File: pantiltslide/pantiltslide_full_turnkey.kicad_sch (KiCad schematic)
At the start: 57 parts, among them J1 Conn_01x22_Socket, J17 Motor_Slide, J18 Motor_Pan, J19 Motor_Tilt, J2 Conn_01x22_Socket, J20 TCA9548A_Mux, J21 AS5600_Pan, J22 AS5600_Tilt, J23 OLED, J24 TCA9548A_Mux, J26 Limit_Min, J27 Limit_Max, J28 Motor_Aux, J29 Enc_Slide, J30 Enc_Pan, J31 Enc_Tilt, J32 Enc_Aux, J33 Btn_SetKeyframe, J34 Btn_ClearKeyframe, J35 Btn_PlayPause, J36 Btn_Reset, J37 5V_In, J38 24V_In, J41 Aux_Max, U1 tmc2209, U2 tmc2209, U3 tmc2209, U4 tmc2209

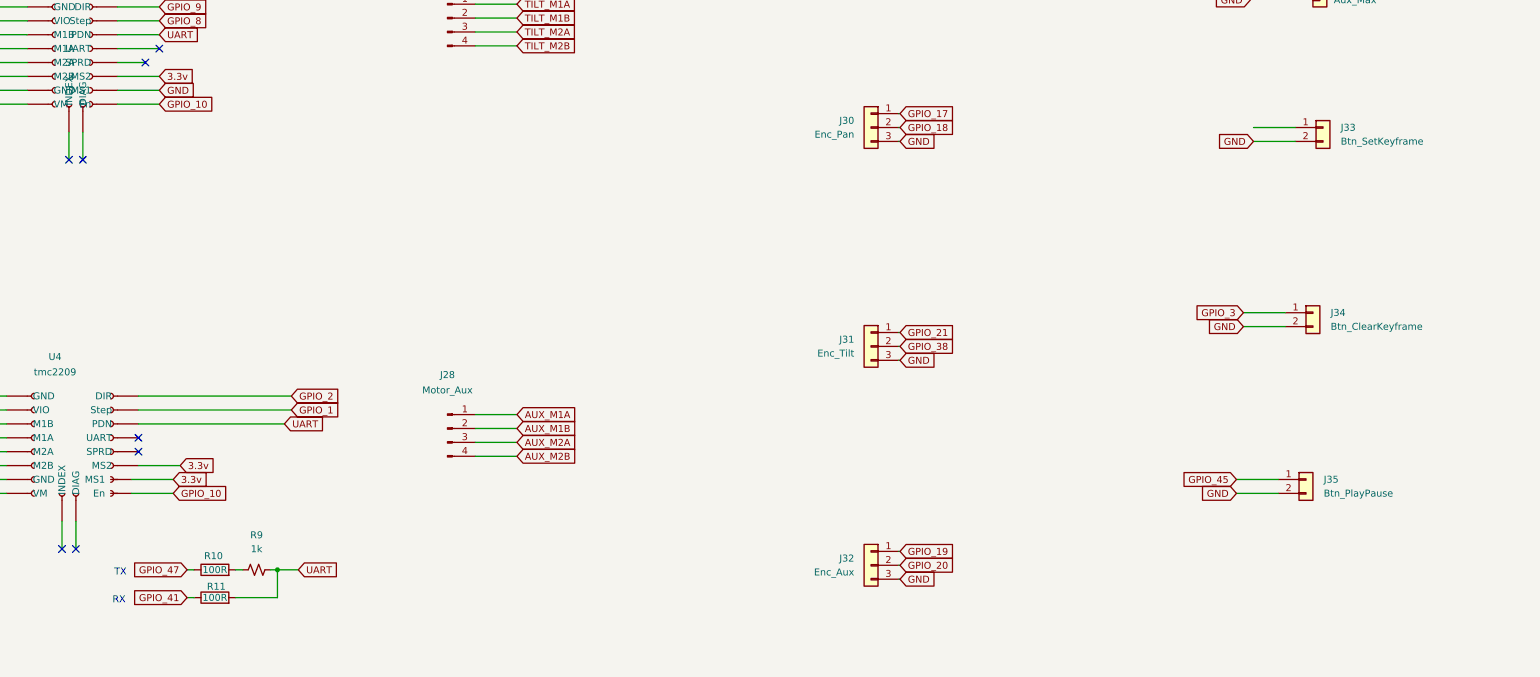
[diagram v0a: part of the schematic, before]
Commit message: more corrections and refinements before prod
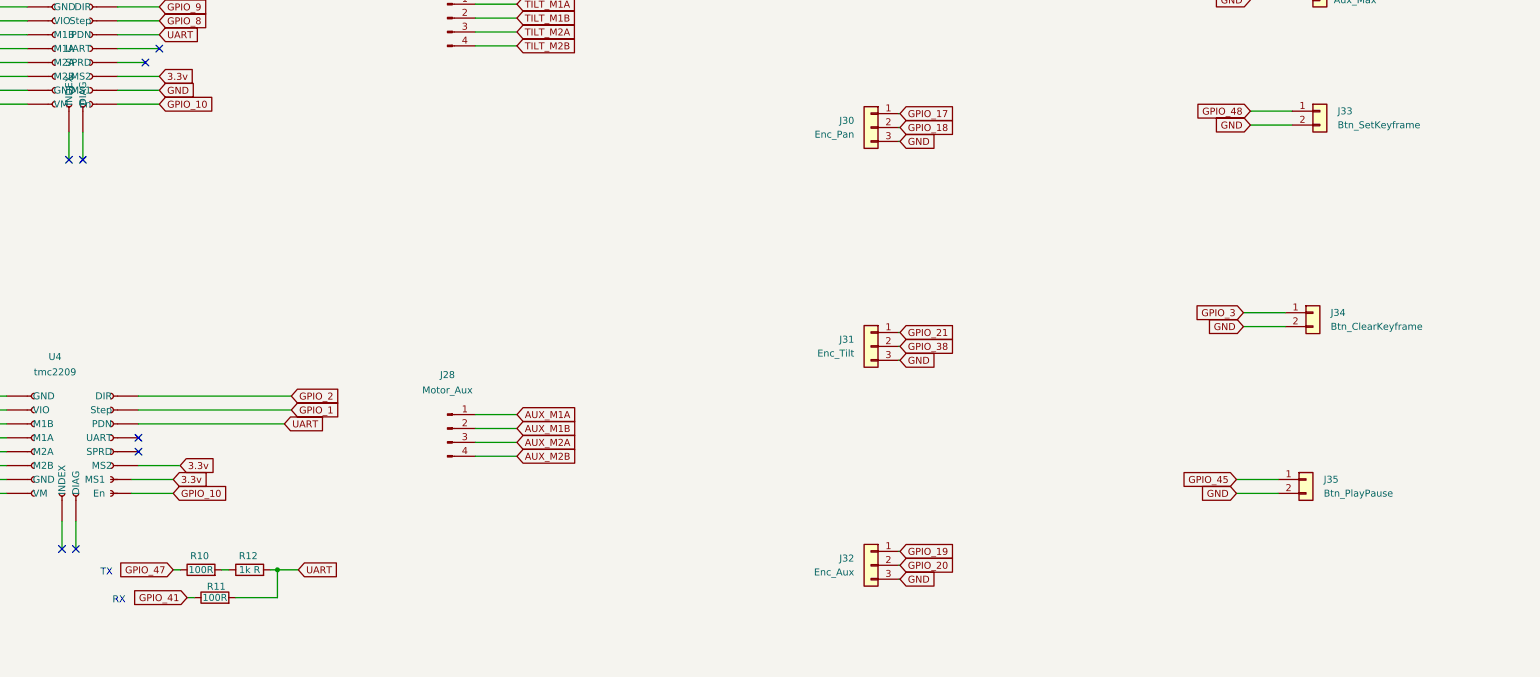
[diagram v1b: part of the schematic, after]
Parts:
- removed R9: 1k, PCM_SparkFun-Resistor:R_0402_1005Metric, symbol PCM_SparkFun-Resistor:1k_0402
- added R12: 1k R, Resistor_SMD:R_0603_1608Metric, symbol Device:R
- R10, R11: footprint (none) -> Resistor_SMD:R_0603_1608Metric
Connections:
- net GPIO_48: now also J33.1 (Pin_1)
- net UART: now also R12.2
- net at R10.2: now also R12.1
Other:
- moved on the sheet: J33, R10
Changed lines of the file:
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@@
 	(text "TX\n"
 		(exclude_from_sim no)
-		(at 300.228 291.338 0)
+		(at 297.688 291.338 0)
 		(effects
 			(font
@@
 	)
 	(junction
+		(at 328.93 290.83)
+		(diameter 0)
+		(color 0 0 0 0)
+	)
+	(junction
 		(at 123.19 345.44)
 		(diameter 0)
@@
 	)
 	(junction
-		(at 328.93 290.83)
-		(diameter 0)
-		(color 0 0 0 0)
-	)
-	(junction
 		(at 59.69 345.44)
 		(diameter 0)
@@
 	(wire
 		(pts
-			(xy 514.92 212.54) (xy 507.3 212.54)
+			(xy 514.35 209.55) (xy 506.73 209.55)
 		)
 		(stroke
@@
 	(wire
 		(pts
-			(xy 514.92 210) (xy 507.3 210)
+			(xy 514.35 207.01) (xy 506.73 207.01)
 		)
 		(stroke
@@
 	(wire
 		(pts
+			(xy 327.66 290.83) (xy 328.93 290.83)
+		)
+		(stroke
+			(width 0)
+			(type default)
+		)
+	)
+	(wire
+		(pts
 			(xy 116.84 96.52) (xy 130.81 96.52)
 		)
@@
 	(wire
 		(pts
+			(xy 318.77 290.83) (xy 320.04 290.83)
+		)
+		(stroke
+			(width 0)
+			(type default)
+		)
+	)
+	(wire
+		(pts
 			(xy 365.08 115) (xy 372.7 115)
 		)
@@
 	(wire
 		(pts
-			(xy 312.42 290.83) (xy 313.69 290.83)
+			(xy 309.88 290.83) (xy 311.15 290.83)
 		)
 		(stroke
@@
 	(wire
 		(pts
-			(xy 322.58 290.83) (xy 321.31 290.83)
-		)
-		(stroke
-			(width 0)
-			(type default)
-		)
-	)
-	(wire
-		(pts
 			(xy 299.72 118.11) (xy 307.34 118.11)
 		)
@@
 		)
 	)
-	(wire
-		(pts
-			(xy 327.66 290.83) (xy 328.93 290.83)
-		)
-		(stroke
-			(width 0)
-			(type default)
-		)
-	)
 	(label "A1"
 		(at 514.35 41.91 180)
@@
 	(global_label "GPIO_47"
 		(shape input)
-		(at 312.42 290.83 180)
+		(at 309.88 290.83 180)
 		(effects
 			(font
@@
 		)
 		(property "Intersheetrefs" "${INTERSHEET_REFS}"
-			(at 312.42 290.83 0)
+			(at 309.88 290.83 0)
 			(hide yes)
 			(show_name no)
@@
 	(global_label "GND"
 		(shape input)
-		(at 507.3 212.54 180)
+		(at 506.73 209.55 180)
 		(effects
 			(font
@@
 		)
 		(property "Intersheetrefs" "${INTERSHEET_REFS}"
-			(at 507.3 212.54 0)
+			(at 506.73 209.55 0)
 			(hide yes)
 			(show_name no)
@@
 		)
 	)
+	(global_label "GPIO_48"
+		(shape input)
+		(at 506.73 207.01 180)
+		(effects
+			(font
+				(size 1.27 1.27)
+			)
+			(justify right)
+		)
+		(property "Intersheetrefs" "${INTERSHEET_REFS}"
+			(at 506.73 207.01 0)
+			(hide yes)
+			(show_name no)
+			(do_not_autoplace no)
+			(effects
+				(font
+					(size 1.27 1.27)
+				)
+			)
+		)
+	)
 	(global_label "MUX_CH4_SCL"
 		(shape input)
@@
 			)
 		)
-		(property "Footprint" ""
+		(property "Footprint" "Resistor_SMD:R_0603_1608Metric"
 			(at 317.5 297.688 90)
 			(hide yes)
@@
 	)
 	(symbol
-		(lib_id "PCM_SparkFun-Resistor:1k_0402")
-		(at 325.12 290.83 0)
-		(unit 1)
-		(body_style 1)
-		(exclude_from_sim no)
-		(in_bom yes)
-		(on_board yes)
-		(in_pos_files yes)
-		(dnp no)
-		(fields_autoplaced yes)
-		(property "Reference" "R9"
-			(at 325.12 284.48 0)
-			(show_name no)
-			(do_not_autoplace no)
-			(effects
-				(font
-					(size 1.27 1.27)
-				)
-			)
-		)
-		(property "Value" "1k"
-			(at 325.12 287.02 0)
-			(show_name no)
-			(do_not_autoplace no)
-			(effects
-				(font
-					(size 1.27 1.27)
-				)
-			)
-		)
-		(property "Footprint" "PCM_SparkFun-Resistor:R_0402_1005Metric"
-			(at 325.12 295.402 0)
-			(hide yes)
-			(show_name no)
-			(do_not_autoplace no)
-			(effects
-				(font
-					(size 1.27 1.27)
-				)
-			)
-		)
-		(property "Datasheet" "https://www.vishay.com/docs/20035/dcrcwe3.pdf"
-			(at 323.85 299.72 0)
-			(hide yes)
-			(show_name no)
-			(do_not_autoplace no)
-			(effects
-				(font
-					(size 1.27 1.27)
-				)
-			)
-		)
-		(property "Description" "Resistor"
-			(at 325.12 302.26 0)
-			(hide yes)
-			(show_name no)
-			(do_not_autoplace no)
-			(effects
-				(font
-					(size 1.27 1.27)
-				)
-			)
-		)
-		(property "PROD_ID" "RES-14342"
-			(at 325.12 297.688 0)
-			(hide yes)
-			(show_name no)
-			(do_not_autoplace no)
-			(effects
-				(font
-					(size 1.27 1.27)
-				)
-			)
-		)
-		(pin "2"
-		)
-		(pin "1"
-		)
-		(instances
-			(project "pantiltslide_full_turnkey"
-				(path "/069dac62-ca78-4a21-b689-b9421532705f"
-					(reference "R9")
-					(unit 1)
-				)
-			)
-		)
-	)
-	(symbol
 		(lib_id "Connector_Generic:Conn_01x03")
 		(at 437.41 170 0)
@@
 	)
 	(symbol
+		(lib_id "Device:R")
+		(at 323.85 290.83 90)
+		(unit 1)
+		(body_style 1)
+		(exclude_from_sim no)
+		(in_bom yes)
+		(on_board yes)
+		(in_pos_files yes)
+		(dnp no)
+		(property "Reference" "R12"
+			(at 323.596 288.29 90)
+			(show_name no)
+			(do_not_autoplace no)
+			(effects
+				(font
+					(size 1.27 1.27)
+				)
+			)
+		)
+		(property "Value" "1k R"
+			(at 323.85 290.83 90)
+			(show_name no)
+			(do_not_autoplace no)
+			(effects
+				(font
+					(size 1.27 1.27)
+				)
+			)
+		)
+		(property "Footprint" "Resistor_SMD:R_0603_1608Metric"
+			(at 323.85 292.608 90)
+			(hide yes)
+			(show_name no)
+			(do_not_autoplace no)
+			(effects
+				(font
+					(size 1.27 1.27)
+				)
+			)
+		)
+		(property "Datasheet" ""
+			(at 323.85 290.83 0)
+			(hide yes)
+			(show_name no)
+			(do_not_autoplace no)
+			(effects
+				(font
+					(size 1.27 1.27)
+				)
+			)
+		)
+		(property "Description" "Resistor"
+			(at 323.85 290.83 0)
+			(hide yes)
+			(show_name no)
+			(do_not_autoplace no)
+			(effects
+				(font
+					(size 1.27 1.27)
+				)
+			)
+		)
+		(pin "1"
+		)
+		(pin "2"
+		)
+		(instances
+			(project "pantiltslide_full_turnkey"
+				(path "/069dac62-ca78-4a21-b689-b9421532705f"
+					(reference "R12")
+					(unit 1)
+				)
+			)
+		)
+	)
+	(symbol
 		(lib_id "power:GND")
 		(at 144.78 382.27 0)
@@
 	(symbol
 		(lib_id "Device:R")
-		(at 317.5 290.83 90)
+		(at 314.96 290.83 90)
 		(unit 1)
 		(body_style 1)
@@
 		(dnp no)
 		(property "Reference" "R10"
-			(at 317.246 288.29 90)
+			(at 314.706 288.29 90)
 			(show_name no)
 			(do_not_autoplace no)
@@
 		)
 		(property "Value" "100R"
-			(at 317.5 290.83 90)
+			(at 314.96 290.83 90)
 			(show_name no)
 			(do_not_autoplace no)
@@
 			)
 		)
-		(property "Footprint" ""
-			(at 317.5 292.608 90)
+		(property "Footprint" "Resistor_SMD:R_0603_1608Metric"
+			(at 314.96 292.608 90)
 			(hide yes)
 			(show_name no)
@@
 		)
 		(property "Datasheet" ""
-			(at 317.5 290.83 0)
+			(at 314.96 290.83 0)
 			(hide yes)
 			(show_name no)
@@
 		)
 		(property "Description" "Resistor"
-			(at 317.5 290.83 0)
+			(at 314.96 290.83 0)
 			(hide yes)
 			(show_name no)
@@
 	(symbol
 		(lib_id "Connector_Generic:Conn_01x02")
-		(at 520 210 0)
+		(at 519.43 207.01 0)
 		(unit 1)
 		(body_style 1)
@@
 		(fields_autoplaced yes)
 		(property "Reference" "J33"
-			(at 523.24 209.9999 0)
+			(at 522.67 207.0099 0)
 			(show_name no)
 			(do_not_autoplace no)
@@
 		)
 		(property "Value" "Btn_SetKeyframe"
-			(at 523.24 212.5399 0)
+			(at 522.67 209.5499 0)
 			(show_name no)
 			(do_not_autoplace no)
@@
 		)
 		(property "Footprint" "Connector_JST:JST_XH_B2B-XH-A_1x02_P2.50mm_Vertical"
-			(at 520 210 0)
+			(at 519.43 207.01 0)
 			(hide yes)
 			(show_name no)
@@
 		)
 		(property "Datasheet" ""
-			(at 520 210 0)
+			(at 519.43 207.01 0)
 			(hide yes)
 			(show_name no)
@@
 		)
 		(property "Description" "Generic connector, single row, 01x02, script generated (kicad-library-utils/schlib/autogen/connector/)"
-			(at 520 210 0)
+			(at 519.43 207.01 0)
 			(hide yes)
 			(show_name no)
